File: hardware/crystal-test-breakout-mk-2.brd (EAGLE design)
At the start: 21.3 x 22.9 mm, 11 parts, among them Q1 1N3904

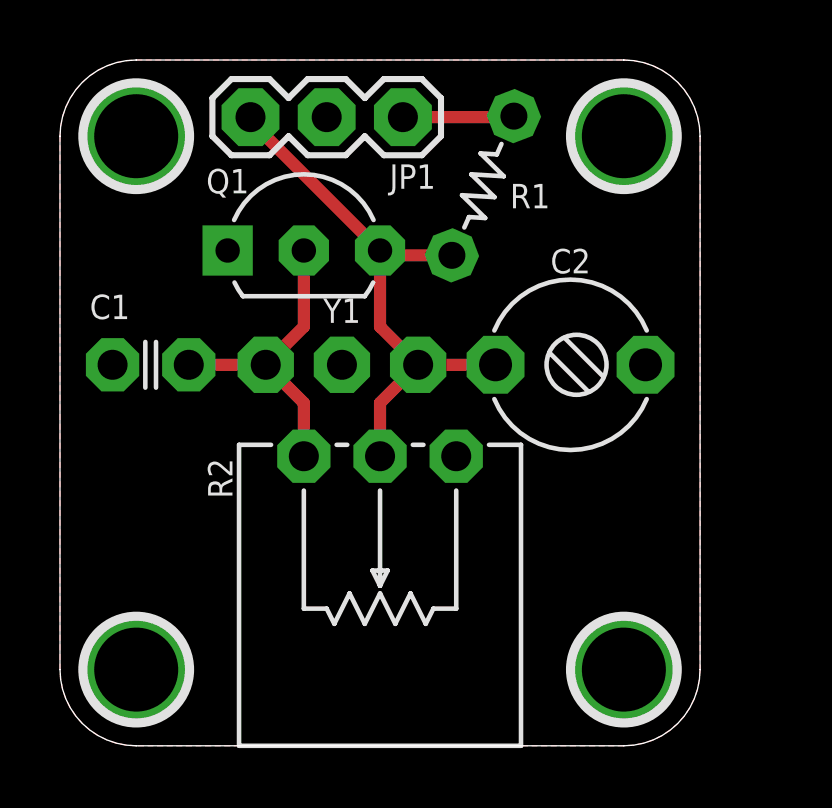
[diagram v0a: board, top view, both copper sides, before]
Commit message: klasdjcvkilasdjfl
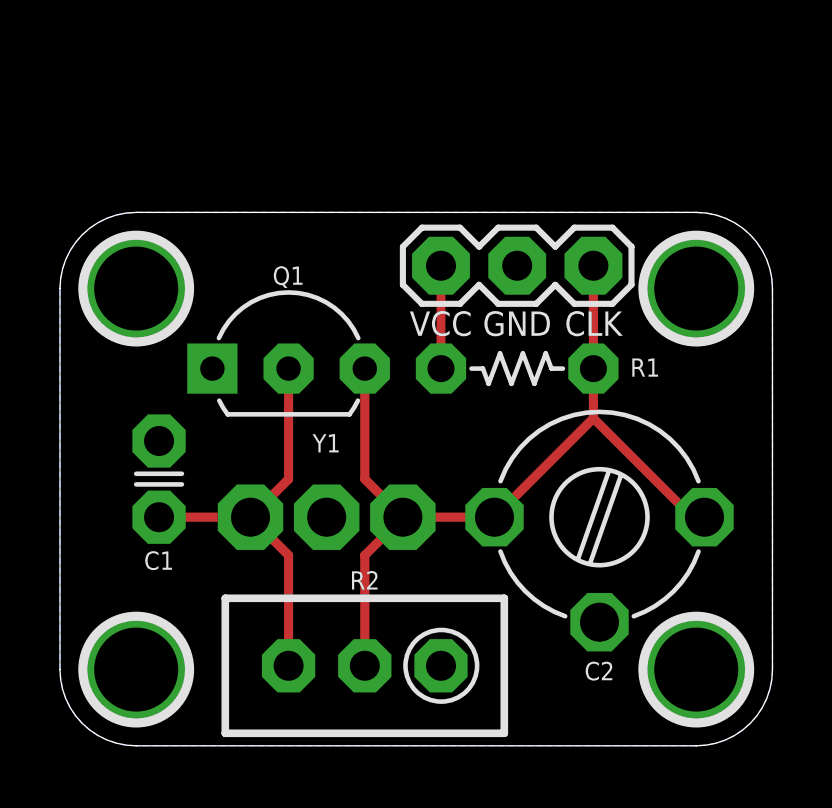
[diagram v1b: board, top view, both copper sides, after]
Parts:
- added U$1: (no value), A_butts:CC-BY-SA-4.0-NO-URL
- C2: device A_butts:CTRIM3050.504 -> A_butts:CTRIM3040.427
- R2: device A_butts:RTRIM3296W-SIDEWAYS -> A_butts:RTRIM3296W
- Y1: device A_butts:RESONATOR-PTH -> A_butts:RESONATOR-PTH-BIGHOLES
- moved R2 7.00 mm to (10.2, 2.67)
- moved R1 6.20 mm to (15.2, 12.6), turned to 180 degrees
- moved H2 5.62 mm to (21.2, 15.2)
- moved C2 5.17 mm to (18.0, 7.62)
- moved JP1 5.11 mm to (12.7, 16.0), turned to 0 degrees
- moved Y1 5.11 mm to (8.89, 7.62)
- moved H1 5.08 mm to (2.54, 15.2)
- moved Q1 3.97 mm to (7.62, 12.6)
- moved C1 3.82 mm to (3.30, 8.89), turned to 90 degrees
- moved H4 2.41 mm to (21.2, 2.54)
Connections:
- net N$4: now also C2.1A, C2.1B; no longer C2.1
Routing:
- net N$4: track 19.3 -> 28.8 mm
- net N$1: track 10.5 -> 14.0 mm
- added copper zone on layer 16, net GND
- removed copper zone on layer 1, net GND
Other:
- board size 21.3 x 22.9 mm -> 23.7 x 17.8 mm
- board text added: "CLK"
- board text added: "Crystal Tester Breakout Revision 1.0"
- board text added: "GND"
- board text added: "VCC"
